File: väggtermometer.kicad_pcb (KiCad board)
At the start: 2 copper layers, 35 x 191 mm, 155 parts, among them J1 USB_C_Receptacle_USB2.0, J2 Conn_01x08, J4 NC, J8 Conn_01x02, Q1 BSS84, SW1 SW_MEC_5G, SW3 SW_MEC_5G, U1 ESP32-C3, U2 RT9080, U3 TC1047AxNB, U4 MCP73831, Y1 Crystal

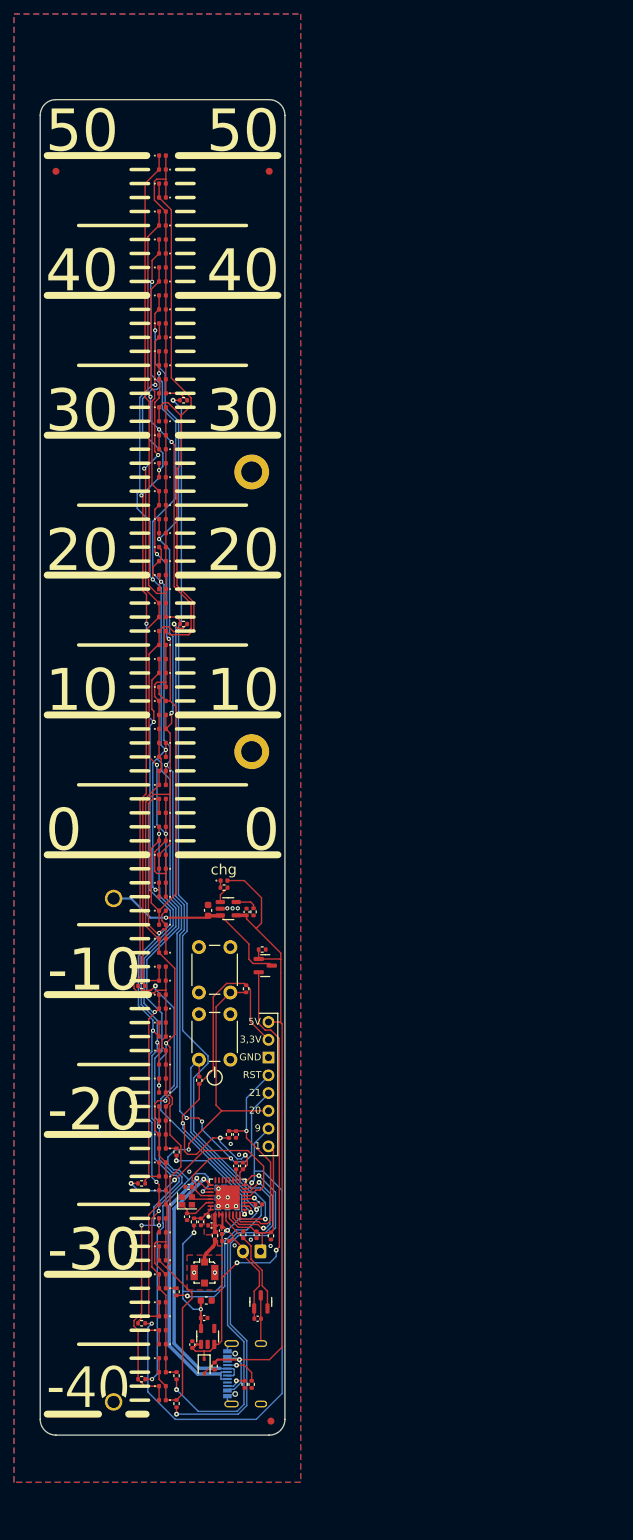
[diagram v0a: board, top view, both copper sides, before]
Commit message: info and stuff
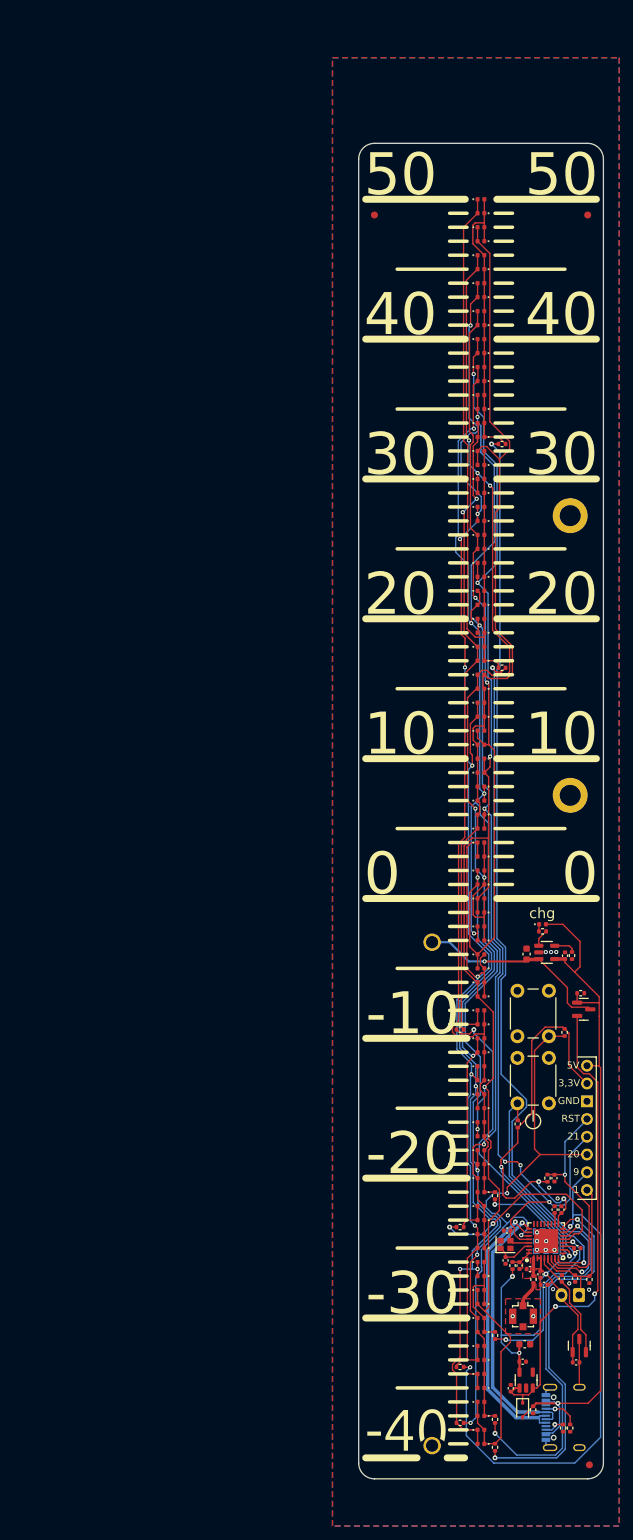
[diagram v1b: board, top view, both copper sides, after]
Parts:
- moved C16 46.0 mm to (115.4, 214.8)
- moved J1 46.0 mm to (114.8, 222.7)
- moved R5 46.0 mm to (113.5, 224.2)
- moved R6 46.0 mm to (114.5, 224.2)
- moved U4 46.0 mm to (111.2, 156.2)
- moved C15 46.0 mm to (108.3, 156.4)
- moved C5 46.0 mm to (105.5, 196.0)
- moved ? 46.0 mm to (117.5, 216.2)
- moved ? 46.0 mm to (112.8, 212.9)
- moved BT1 46.0 mm to (94.8, 154.8)
- moved C1 46.0 mm to (107.3, 201.0)
- moved C10 46.0 mm to (115.6, 198.5)
- moved C11 46.0 mm to (106.0, 218.6)
- moved C12 46.0 mm to (107.8, 214.8)
- moved C13 46.0 mm to (110.8, 203.8)
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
